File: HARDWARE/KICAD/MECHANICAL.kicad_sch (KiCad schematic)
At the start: 7 parts

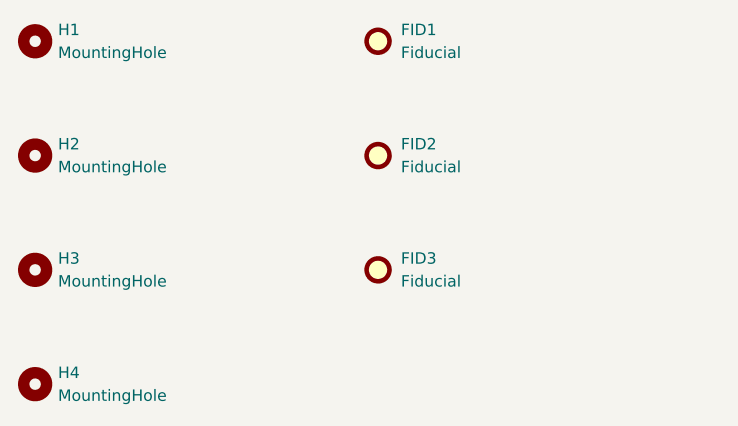
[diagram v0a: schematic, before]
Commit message: Finished Revision 0 design. Used plugin to make manufacturing files. Purchased 5 units in JLCPCB. Let's wait to check the results! :D
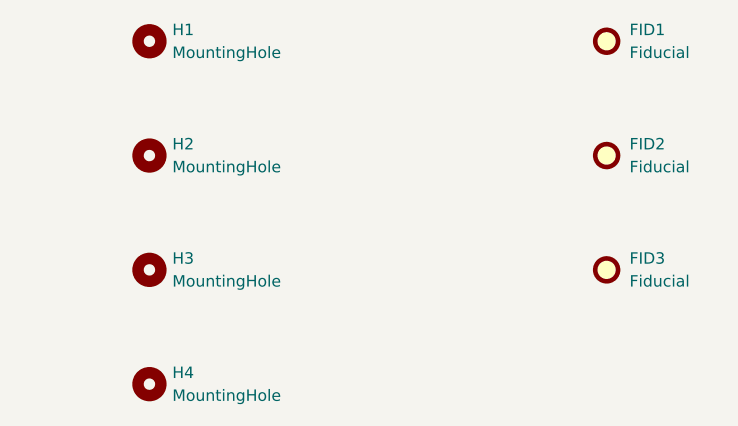
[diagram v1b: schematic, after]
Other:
- title: STM32 EXPLORER BOARD -> STM32 EXPLORER BOARD PROTOTYPE
- moved on the sheet: FID1, FID2, FID3, H1, H2, H3, H4
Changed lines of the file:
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@@
 	(paper "A4")
 	(title_block
-		(title "STM32 EXPLORER BOARD")
-		(date "2024-04-26")
+		(title "STM32 EXPLORER BOARD PROTOTYPE")
+		(date "2024-07-21")
 		(rev "00")
 		(company "Mechatronix Lab")
@@
 	(symbol
 		(lib_id "Mechanical:Fiducial")
-		(at 139.7 101.6 0)
+		(at 165.1 101.6 0)
 		(unit 1)
 		(exclude_from_sim no)
@@
 		(fields_autoplaced yes)
 		(property "Reference" "FID3"
-			(at 142.24 100.3299 0)
+			(at 167.64 100.3299 0)
 			(effects
 				(font
@@
 		)
 		(property "Value" "Fiducial"
-			(at 142.24 102.8699 0)
+			(at 167.64 102.8699 0)
 			(effects
 				(font
@@
 		)
 		(property "Footprint" "Fiducial:Fiducial_0.75mm_Mask1.5mm"
-			(at 139.7 101.6 0)
-			(effects
-				(font
-					(size 1.27 1.27)
-				)
-				(hide yes)
-			)
-		)
-		(property "Datasheet" "~"
-			(at 139.7 101.6 0)
+			(at 165.1 101.6 0)
+			(effects
+				(font
+					(size 1.27 1.27)
+				)
+				(hide yes)
+			)
+		)
+		(property "Datasheet" "~"
+			(at 165.1 101.6 0)
 			(effects
 				(font
@@
 		)
 		(property "Description" "Fiducial Marker"
-			(at 139.7 101.6 0)
+			(at 165.1 101.6 0)
 			(effects
 				(font
@@
 	(symbol
 		(lib_id "Mechanical:MountingHole")
-		(at 101.6 76.2 0)
+		(at 114.3 76.2 0)
 		(unit 1)
 		(exclude_from_sim no)
@@
 		(fields_autoplaced yes)
 		(property "Reference" "H1"
-			(at 104.14 74.9299 0)
+			(at 116.84 74.9299 0)
 			(effects
 				(font
@@
 		)
 		(property "Value" "MountingHole"
-			(at 104.14 77.4699 0)
+			(at 116.84 77.4699 0)
 			(effects
 				(font
@@
 		)
 		(property "Footprint" "MountingHole:MountingHole_3.2mm_M3"
-			(at 101.6 76.2 0)
-			(effects
-				(font
-					(size 1.27 1.27)
-				)
-				(hide yes)
-			)
-		)
-		(property "Datasheet" "~"
-			(at 101.6 76.2 0)
+			(at 114.3 76.2 0)
+			(effects
+				(font
+					(size 1.27 1.27)
+				)
+				(hide yes)
+			)
+		)
+		(property "Datasheet" "~"
+			(at 114.3 76.2 0)
 			(effects
 				(font
@@
 		)
 		(property "Description" "Mounting Hole without connection"
-			(at 101.6 76.2 0)
+			(at 114.3 76.2 0)
 			(effects
 				(font
@@
 	(symbol
 		(lib_id "Mechanical:Fiducial")
-		(at 139.7 76.2 0)
+		(at 165.1 76.2 0)
 		(unit 1)
 		(exclude_from_sim no)
@@
 		(fields_autoplaced yes)
 		(property "Reference" "FID1"
-			(at 142.24 74.9299 0)
+			(at 167.64 74.9299 0)
 			(effects
 				(font
@@
 		)
 		(property "Value" "Fiducial"
-			(at 142.24 77.4699 0)
+			(at 167.64 77.4699 0)
 			(effects
 				(font
@@
 		)
 		(property "Footprint" "Fiducial:Fiducial_0.75mm_Mask1.5mm"
-			(at 139.7 76.2 0)
-			(effects
-				(font
-					(size 1.27 1.27)
-				)
-				(hide yes)
-			)
-		)
-		(property "Datasheet" "~"
-			(at 139.7 76.2 0)
+			(at 165.1 76.2 0)
+			(effects
+				(font
+					(size 1.27 1.27)
+				)
+				(hide yes)
+			)
+		)
+		(property "Datasheet" "~"
+			(at 165.1 76.2 0)
 			(effects
 				(font
@@
 		)
 		(property "Description" "Fiducial Marker"
-			(at 139.7 76.2 0)
+			(at 165.1 76.2 0)
 			(effects
 				(font
@@
 	(symbol
 		(lib_id "Mechanical:Fiducial")
-		(at 139.7 88.9 0)
+		(at 165.1 88.9 0)
 		(unit 1)
 		(exclude_from_sim no)
@@
 		(fields_autoplaced yes)
 		(property "Reference" "FID2"
-			(at 142.24 87.6299 0)
+			(at 167.64 87.6299 0)
 			(effects
 				(font
@@
 		)
 		(property "Value" "Fiducial"
-			(at 142.24 90.1699 0)
+			(at 167.64 90.1699 0)
 			(effects
 				(font
@@
 		)
 		(property "Footprint" "Fiducial:Fiducial_0.75mm_Mask1.5mm"
-			(at 139.7 88.9 0)
-			(effects
-				(font
-					(size 1.27 1.27)
-				)
-				(hide yes)
-			)
-		)
-		(property "Datasheet" "~"
-			(at 139.7 88.9 0)
+			(at 165.1 88.9 0)
+			(effects
+				(font
+					(size 1.27 1.27)
+				)
+				(hide yes)
+			)
+		)
+		(property "Datasheet" "~"
+			(at 165.1 88.9 0)
 			(effects
 				(font
@@
 		)
 		(property "Description" "Fiducial Marker"
-			(at 139.7 88.9 0)
+			(at 165.1 88.9 0)
 			(effects
 				(font
@@
 	(symbol
 		(lib_id "Mechanical:MountingHole")
-		(at 101.6 88.9 0)
+		(at 114.3 88.9 0)
 		(unit 1)
 		(exclude_from_sim no)
@@
 		(fields_autoplaced yes)
 		(property "Reference" "H2"
-			(at 104.14 87.6299 0)
+			(at 116.84 87.6299 0)
 			(effects
 				(font
@@
 		)
 		(property "Value" "MountingHole"
-			(at 104.14 90.1699 0)
+			(at 116.84 90.1699 0)
 			(effects
 				(font
@@
 		)
 		(property "Footprint" "MountingHole:MountingHole_3.2mm_M3"
-			(at 101.6 88.9 0)
-			(effects
-				(font
-					(size 1.27 1.27)
-				)
-				(hide yes)
-			)
-		)
-		(property "Datasheet" "~"
-			(at 101.6 88.9 0)
+			(at 114.3 88.9 0)
+			(effects
+				(font
+					(size 1.27 1.27)
+				)
+				(hide yes)
+			)
+		)
+		(property "Datasheet" "~"
+			(at 114.3 88.9 0)
 			(effects
 				(font
@@
 		)
 		(property "Description" "Mounting Hole without connection"
-			(at 101.6 88.9 0)
+			(at 114.3 88.9 0)
 			(effects
 				(font
@@
 	(symbol
 		(lib_id "Mechanical:MountingHole")
-		(at 101.6 114.3 0)
+		(at 114.3 114.3 0)
 		(unit 1)
 		(exclude_from_sim no)
@@
 		(fields_autoplaced yes)
 		(property "Reference" "H4"
-			(at 104.14 113.0299 0)
+			(at 116.84 113.0299 0)
 			(effects
 				(font
@@
 		)
 		(property "Value" "MountingHole"
-			(at 104.14 115.5699 0)
+			(at 116.84 115.5699 0)
 			(effects
 				(font
@@
 		)
 		(property "Footprint" "MountingHole:MountingHole_3.2mm_M3"
-			(at 101.6 114.3 0)
-			(effects
-				(font
-					(size 1.27 1.27)
-				)
-				(hide yes)
-			)
-		)
-		(property "Datasheet" "~"
-			(at 101.6 114.3 0)
+			(at 114.3 114.3 0)
+			(effects
+				(font
+					(size 1.27 1.27)
+				)
+				(hide yes)
+			)
+		)
+		(property "Datasheet" "~"
+			(at 114.3 114.3 0)
 			(effects
 				(font
@@
 		)
 		(property "Description" "Mounting Hole without connection"
-			(at 101.6 114.3 0)
+			(at 114.3 114.3 0)
 			(effects
 				(font
@@
 	(symbol
 		(lib_id "Mechanical:MountingHole")
-		(at 101.6 101.6 0)
+		(at 114.3 101.6 0)
 		(unit 1)
 		(exclude_from_sim no)
@@
 		(fields_autoplaced yes)
 		(property "Reference" "H3"
-			(at 104.14 100.3299 0)
+			(at 116.84 100.3299 0)
 			(effects
 				(font
@@
 		)
 		(property "Value" "MountingHole"
-			(at 104.14 102.8699 0)
+			(at 116.84 102.8699 0)
 			(effects
 				(font
@@
 		)
 		(property "Footprint" "MountingHole:MountingHole_3.2mm_M3"
-			(at 101.6 101.6 0)
-			(effects
-				(font
-					(size 1.27 1.27)
-				)
-				(hide yes)
-			)
-		)
-		(property "Datasheet" "~"
-			(at 101.6 101.6 0)
+			(at 114.3 101.6 0)
+			(effects
+				(font
+					(size 1.27 1.27)
+				)
+				(hide yes)
+			)
+		)
+		(property "Datasheet" "~"
+			(at 114.3 101.6 0)
 			(effects
 				(font
@@
 		)
 		(property "Description" "Mounting Hole without connection"
-			(at 101.6 101.6 0)
-			(effects
-				(font
+			(at 114.3 101.6 0)
+			(effects
+				(font
